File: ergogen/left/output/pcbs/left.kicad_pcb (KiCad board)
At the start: 2 copper layers, 163.2 x 111 mm, 45 parts

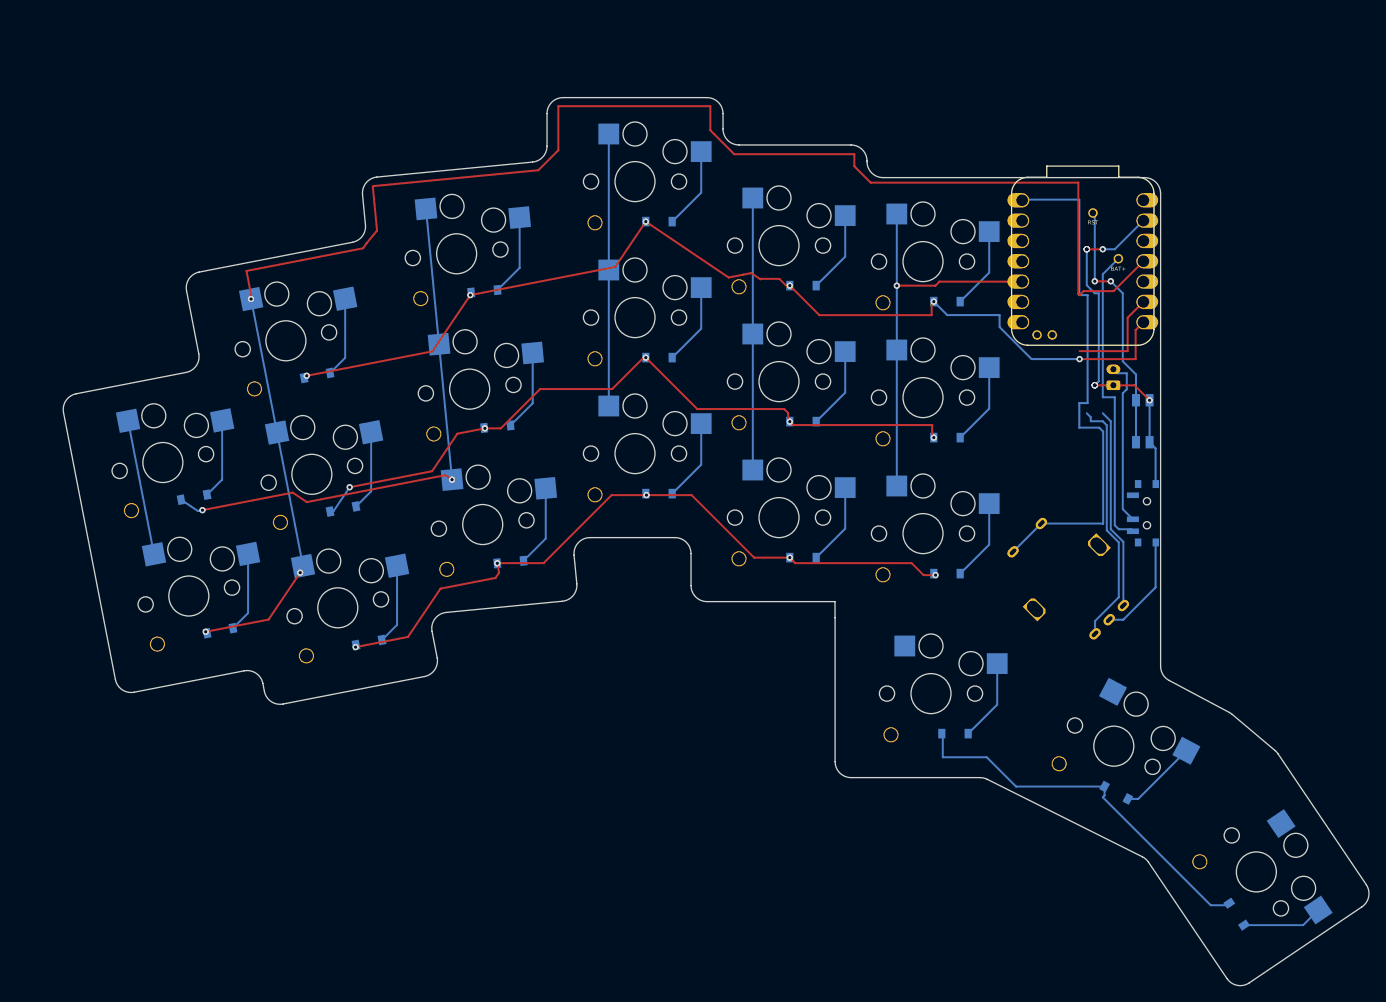
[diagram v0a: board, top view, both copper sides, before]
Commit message: t
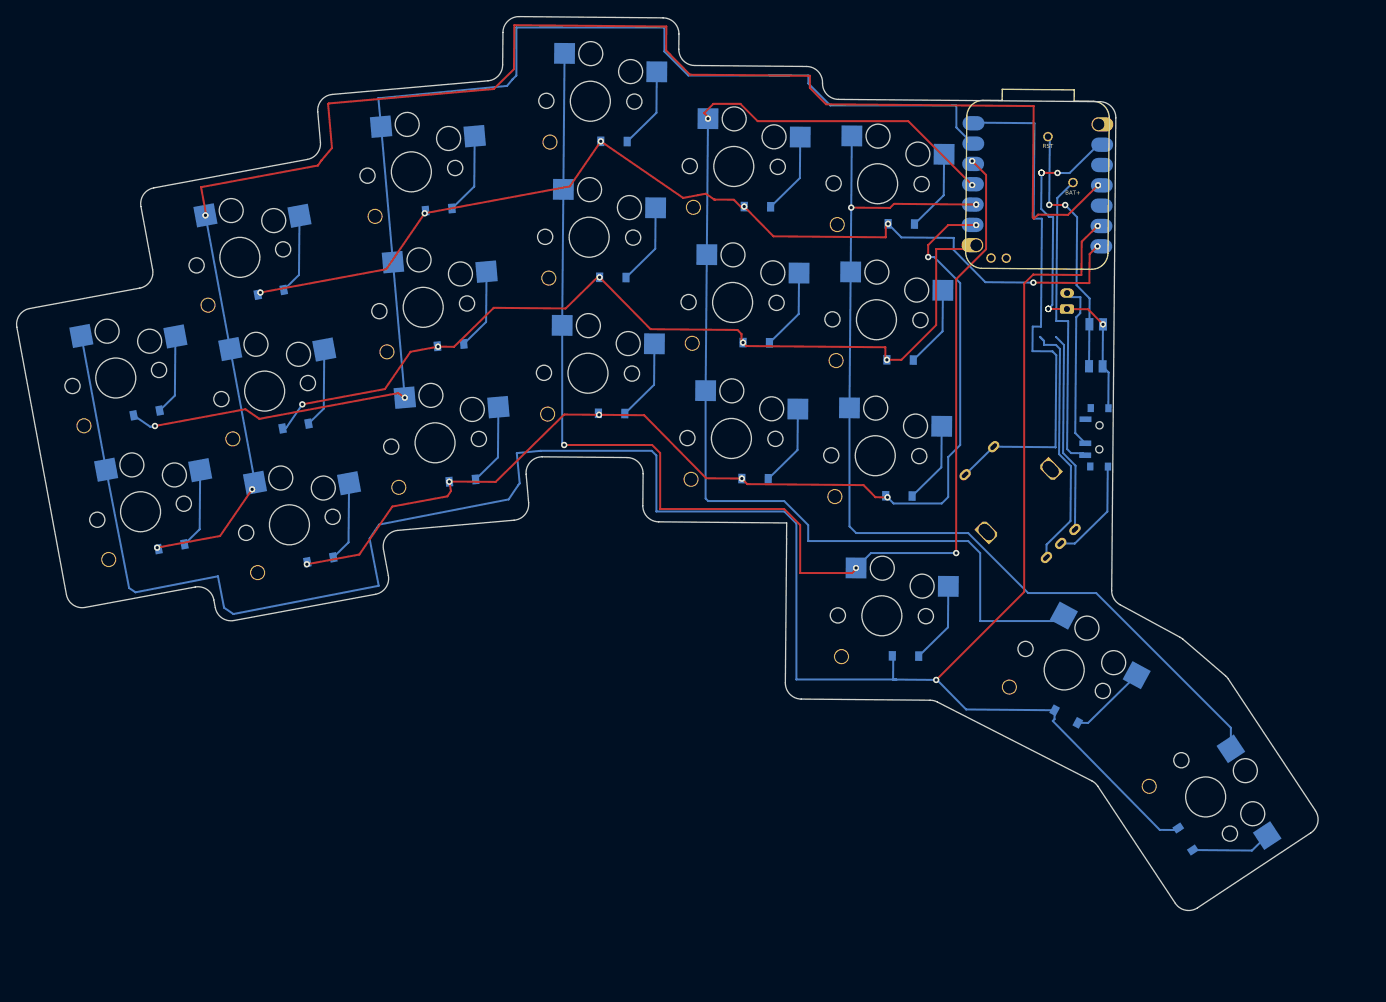
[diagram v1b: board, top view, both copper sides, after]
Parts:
- moved S19 12.1 mm to (62.0, 75.3), turned to 10.5 degrees
- moved D19 12.1 mm to (65.9, 79.7), turned to 10.5 degrees
- moved S20 12.1 mm to (58.9, 58.6), turned to 10.5 degrees
- moved D20 12.1 mm to (62.8, 63.0), turned to 10.5 degrees
- moved S1 12.0 mm to (80.7, 77.0), turned to 10.5 degrees
- moved D1 12.0 mm to (84.5, 81.3), turned to 10.5 degrees
- moved S2 12.0 mm to (77.6, 60.3), turned to 10.5 degrees
- moved D2 11.9 mm to (81.4, 64.6), turned to 10.5 degrees
- moved S3 11.9 mm to (74.5, 43.5), turned to 10.5 degrees
- moved D3 11.9 mm to (78.3, 47.9), turned to 10.5 degrees
- moved S4 11.8 mm to (98.9, 66.7), turned to 5 degrees
- moved D4 11.8 mm to (102.3, 71.4), turned to 5 degrees
- moved S5 11.8 mm to (97.4, 49.8), turned to 5 degrees
- moved D5 11.8 mm to (100.8, 54.5), turned to 5 degrees
- moved S6 11.7 mm to (95.9, 32.8), turned to 5 degrees
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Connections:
- U? pad GND: GND -> (no net)
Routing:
- net P8: track 78.1 -> 289.9 mm, vias 0 -> 2
- net P2: track 34.0 -> 164.9 mm, vias 0 -> 4
- net P3: track 34.0 -> 144.7 mm, vias 0 -> 2
- net P1: track 71.7 -> 166.7 mm
- net P4: track 49.9 -> 125.5 mm, vias 1 -> 2
- net P5: track 86.0 -> 135.5 mm, vias 5 -> 7
- net P6: track 89.1 -> 111.8 mm
- net RE_A: track 31.3 -> 32.1 mm
- net P0: vias 3 -> 4
- net P7: vias 6 -> 7
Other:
- board size 163.2 x 111 mm -> 162.7 x 111.7 mm

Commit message: right side development
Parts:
- moved D19 101.2 mm to (140.8, 147.7), turned to 11 degrees
- moved S19 101.2 mm to (136.9, 143.4), turned to 11 degrees
- moved D20 101.1 mm to (137.6, 131.0), turned to 11 degrees
- moved S20 101.1 mm to (133.7, 126.7), turned to 11 degrees
- moved D1 101.1 mm to (159.4, 149.2), turned to 11 degrees
- moved S1 101.1 mm to (155.5, 144.9), turned to 11 degrees
- moved D2 101.0 mm to (156.2, 132.5), turned to 11 degrees
- moved S2 101.0 mm to (152.3, 128.2), turned to 11 degrees
- moved D4 100.9 mm to (177.1, 139.1), turned to 5.5 degrees
- moved D3 100.9 mm to (152.9, 115.8), turned to 11 degrees
- moved S4 100.9 mm to (173.6, 134.5), turned to 5.5 degrees
- moved S3 100.9 mm to (149.0, 111.5), turned to 11 degrees
- moved D5 100.8 mm to (175.5, 122.2), turned to 5.5 degrees
- moved S5 100.8 mm to (172.0, 117.5), turned to 5.5 degrees
- moved D7 100.7 mm to (195.7, 130.6), turned to 0 degrees
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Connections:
- RE1 pad : (no net) -> GND
- U? pad : P7 -> P6
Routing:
- net GND: track 58.2 -> 95.4 mm, vias 8 -> 7
- net P10: track 66.3 -> 91.4 mm, vias 0 -> 2
- net P0: track 201.4 -> 184.9 mm
- net P6: track 111.8 -> 124.3 mm, vias 5 -> 6
- net P1: track 166.7 -> 178.3 mm
- net BAT_P: track 38.2 -> 49.1 mm, vias 0 -> 2
- net P3: track 144.7 -> 155.2 mm, vias 2 -> 3
- net RST: track 32.1 -> 41.3 mm
- net P4: track 125.5 -> 133.0 mm
- net P2: track 164.9 -> 158.7 mm, vias 4 -> 6
- net P8: track 289.9 -> 293.4 mm
- net P7: track 126.8 -> 128.5 mm, vias 7 -> 5
- net P5: track 135.5 -> 134.4 mm, vias 7 -> 6
- added copper zone on B.Cu, net GND
- added copper zone on F.Cu, net GND
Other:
- board size 162.7 x 111.7 mm -> 163.2 x 111 mm
